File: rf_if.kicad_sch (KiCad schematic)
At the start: 12 parts, among them U3 Adafruit_Si5351, U4 74LVC74, U5 74HCT244, U6 74HC4066, U7 74HC4066

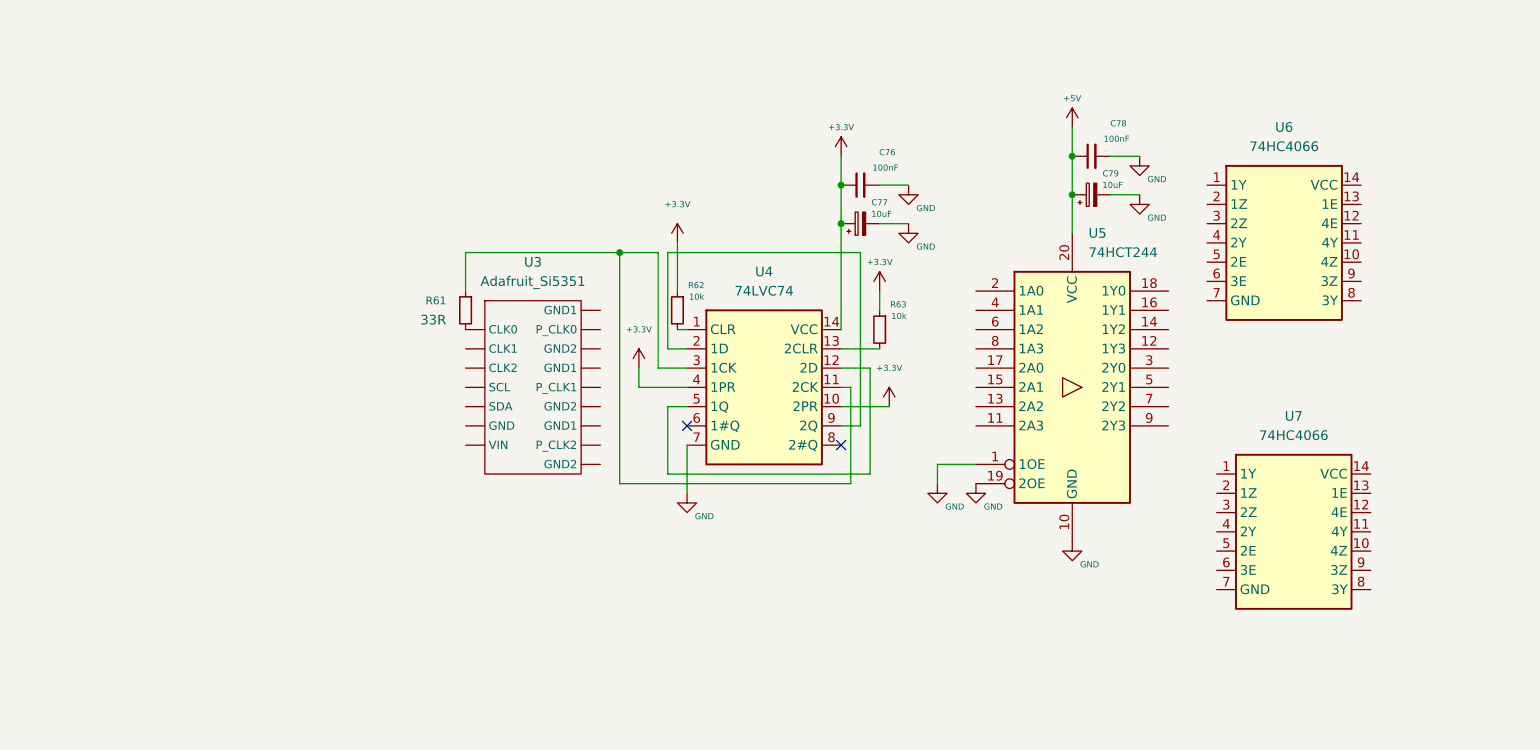
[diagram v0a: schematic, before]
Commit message: Logical Work, Mixers
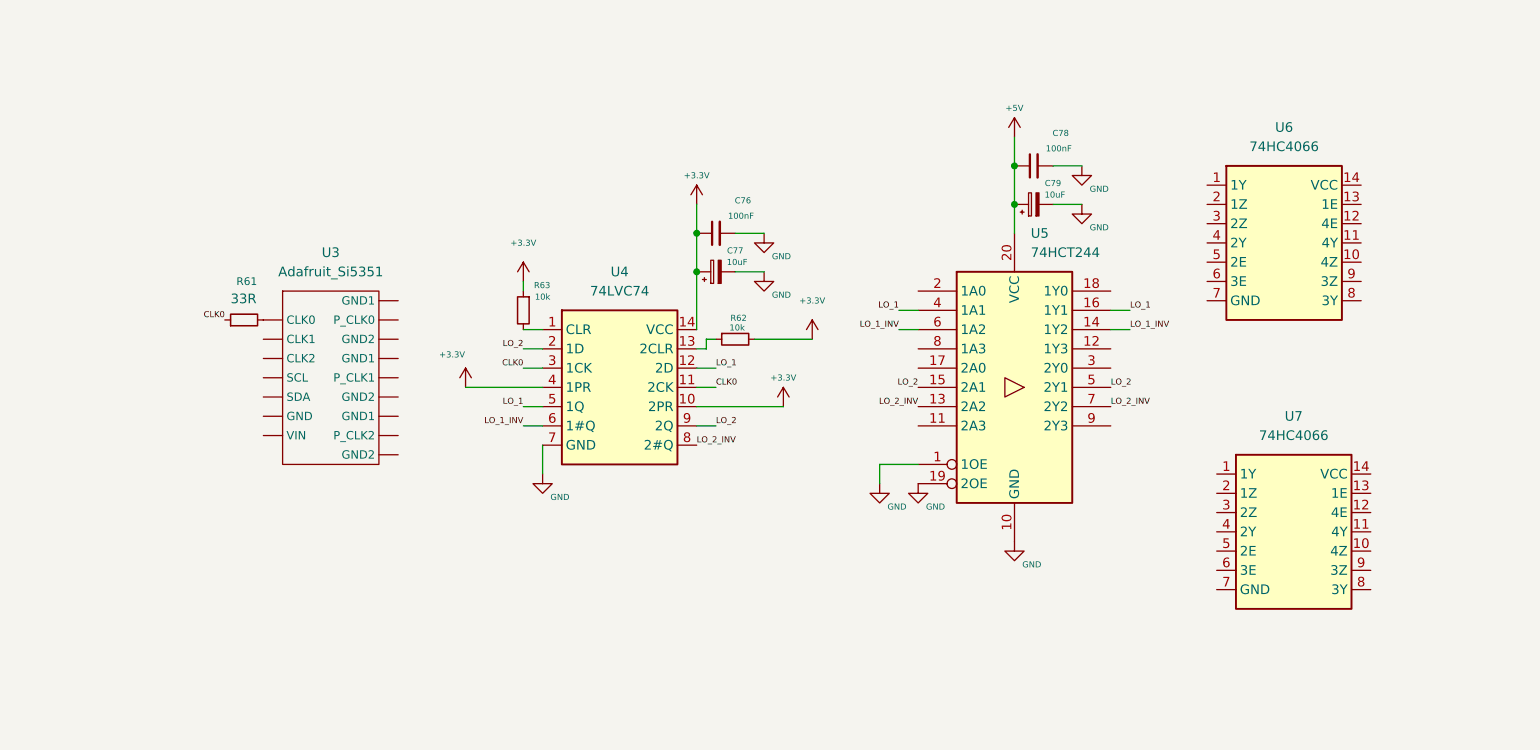
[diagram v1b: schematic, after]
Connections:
- net +3.3V: now also R62.2; no longer R62.1
- net at R63.2: now also U4.1 (CLR); no longer U4.13 (2CLR)
- net CLK0: now reaches R61.1, U4.11 (2CK), U4.3 (1CK)
- net LO_1: now reaches U4.12 (2D), U4.5 (1Q)
- net LO_1: now also U5.16 (1Y1), U5.4 (1A1)
- net LO_2: now reaches U4.2 (1D), U4.9 (2Q)
- net LO_2: now also U5.15 (2A1), U5.5 (2Y1)
- net LO_1_INV: now reaches U4.6 (1#Q)
- net LO_1_INV: now also U5.14 (1Y2), U5.6 (1A2)
- net LO_2_INV: now reaches U4.8 (2#Q)
- net LO_2_INV: now also U5.13 (2A2), U5.7 (2Y2)
- new net: R62.1, U4.13 (2CLR)
- no-connect marks 2 -> 0
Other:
- moved on the sheet: C76, C77, C78, C79, R61, R62, R63, U3, U4, U5

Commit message: Logical Work, Mixers II
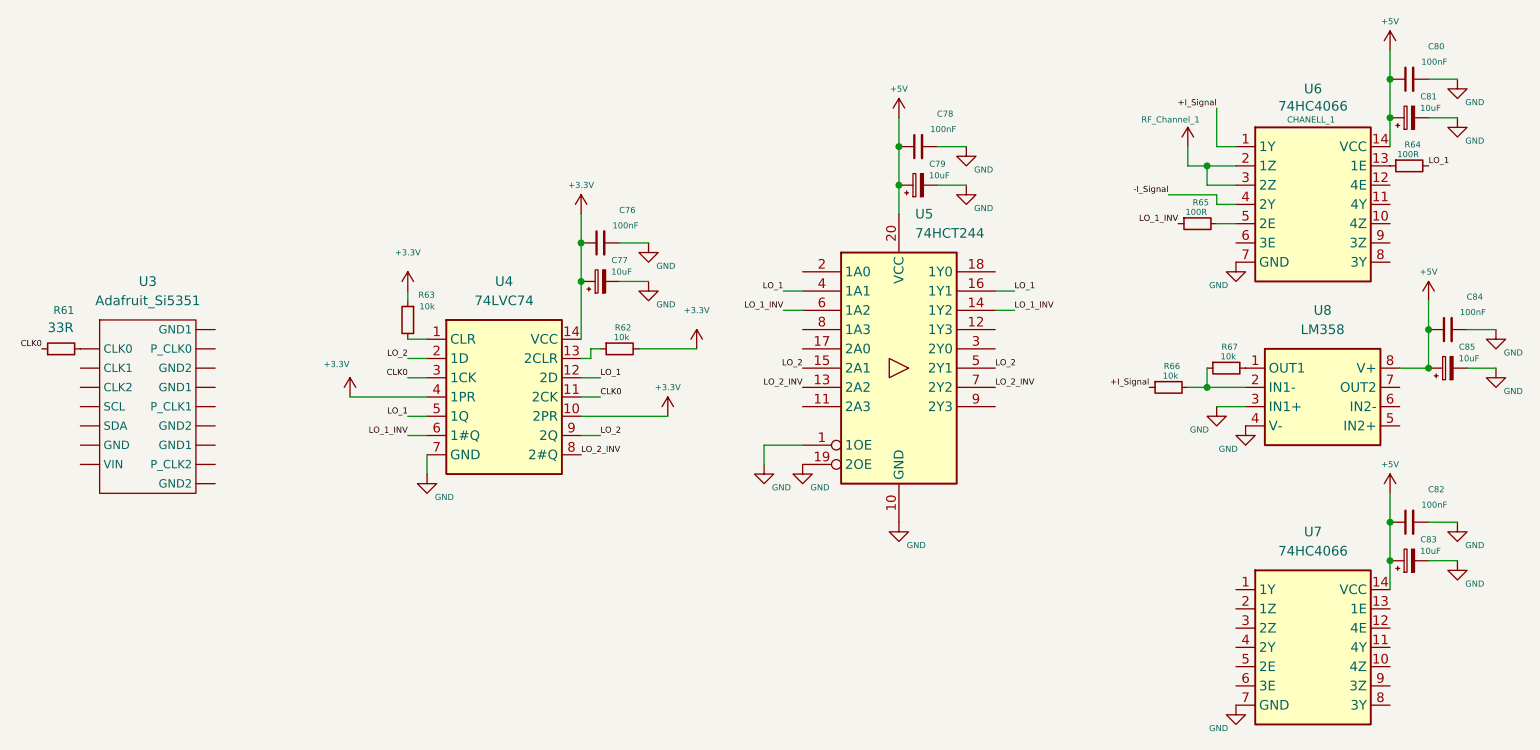
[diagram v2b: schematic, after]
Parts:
- added C80, C82, C84: 100nF, symbol Device:C_Small
- added C81, C83, C85: 10uF, symbol Device:C_Polarized_Small
- added R64, R65: 100R, symbol Device:R_Small
- added R66, R67: 10k, symbol Device:R_Small
- added U8: LM358, symbol omega:LM358
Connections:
- net +5V: now also U6.14 (VCC), U7.14 (VCC), C80.1, C81.1, C82.1, C83.1, C84.1, C85.1, U8.8 (V+)
- net GND: now also U6.7 (GND), U7.7 (GND), C80.2, C81.2, C82.2, C83.2, C84.2, C85.2, U8.3 (IN1+), U8.4 (V-)
- net LO_1: now also R64.2
- net LO_1_INV: now also R65.1
- net +I_Signal: now reaches U6.1 (1Y)
- net +I_Signal: now also R66.1
- net at U6.13 (1E): now also R64.1
- net RF_Channel_1: now reaches U6.2 (1Z)
- net RF_Channel_1: now also U6.3 (2Z)
- net -I_Signal: now reaches U6.4 (2Y)
- net at U6.5 (2E): now also R65.2
- new net: R66.2, R67.1, U8.2 (IN1-)
- new net: R67.2, U8.1 (OUT1)
- new net: U8.11 (NC), U8.4 (V-)
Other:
- note added: "CHANELL_1"
- moved on the sheet: C76, C77, C78, C79, R61, R62, R63, U3, U4, U5, U6, U7
